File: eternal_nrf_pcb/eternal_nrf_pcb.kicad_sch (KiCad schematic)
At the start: 52 parts, among them J1 Conn_01x05_Pin, Q1 IRLML6244, Q2 IRLML6402, SW1 SW_Push, U1 BQ25504, U2 nRF52810-QCxx, U3 DRV5032DU, U4 SHTC3, Y1 Crystal_GND24

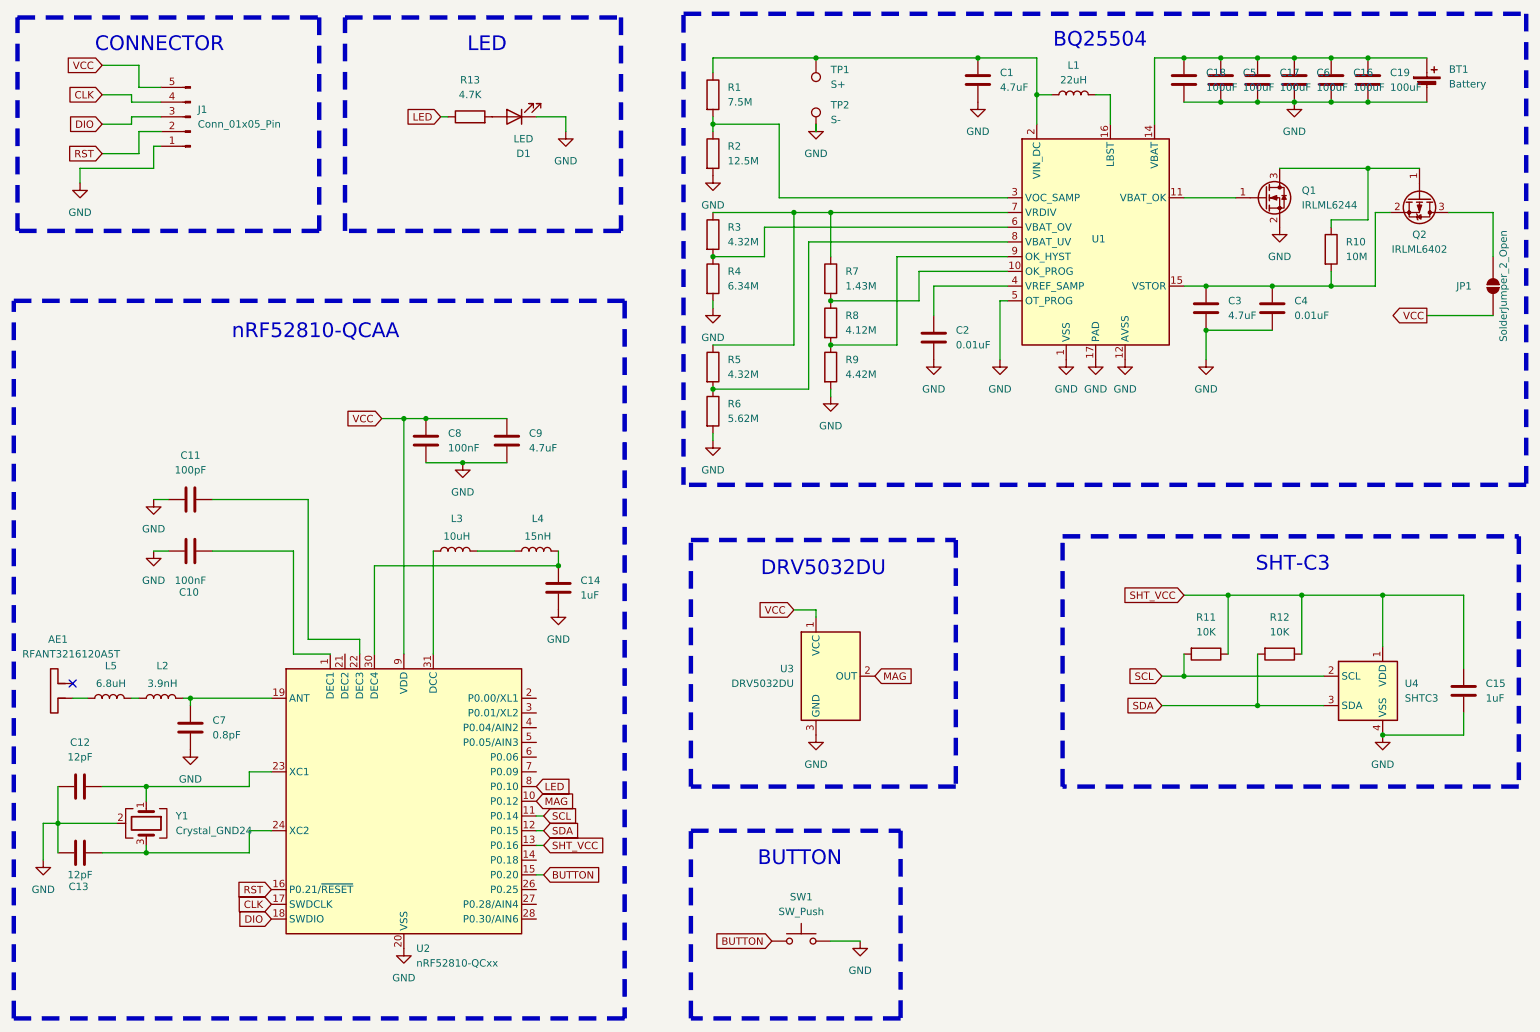
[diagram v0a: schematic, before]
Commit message: complete board
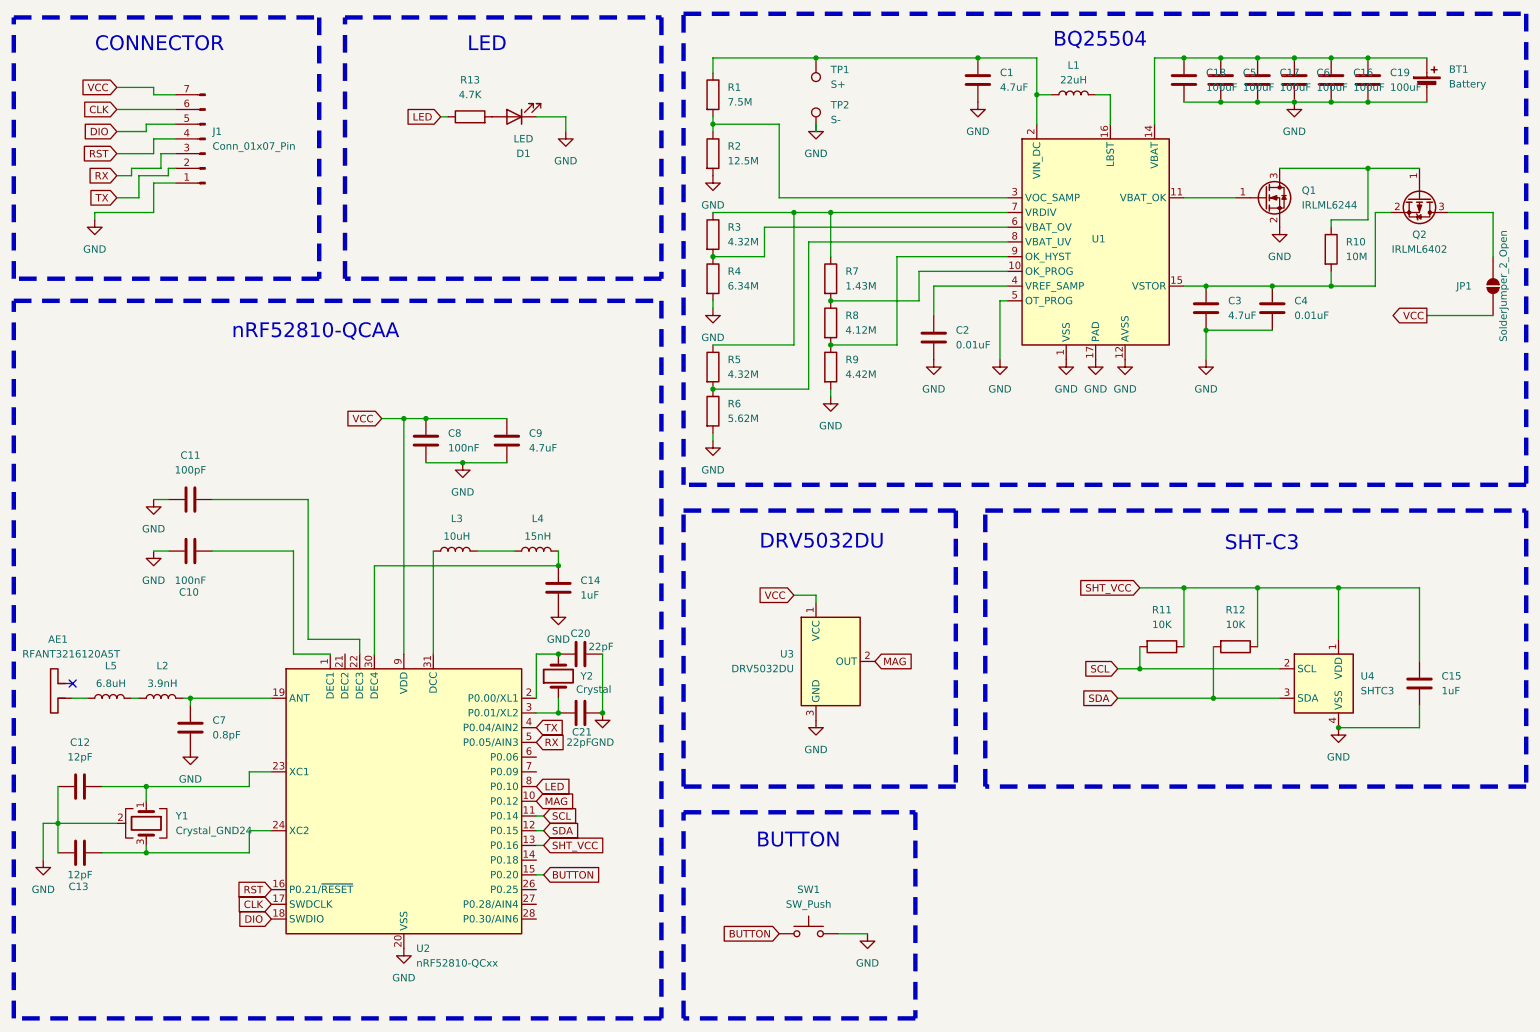
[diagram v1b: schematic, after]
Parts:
- removed J1: Conn_01x05_Pin, Connector_PinHeader_2.54mm:PinHeader_1x05_P2.54mm_Vertical, symbol Connector:Conn_01x05_Pin
- added C20, C21: 22pF, Capacitor_SMD:C_0402_1005Metric_Pad0.74x0.62mm_HandSolder, symbol Device:C
- added J1: Conn_01x07_Pin, Connector_PinHeader_2.54mm:PinHeader_1x07_P2.54mm_Vertical, symbol Connector:Conn_01x07_Pin
- added Y2: Crystal, Crystal:Crystal_SMD_3215-2Pin_3.2x1.5mm, symbol Device:Crystal
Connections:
- net CLK: now also J1.6 (Pin_6)
- net DIO: now also J1.5 (Pin_5)
- net GND: now also C20.1, C21.2, J1.1 (Pin_1)
- net RST: now also J1.4 (Pin_4)
- net VCC: now also J1.7 (Pin_7)
- net at U2.2 (P0.00/XL1): now also C21.1, Y2.2
- net at U2.3 (P0.01/XL2): now also C20.2, Y2.1
- net TX: now reaches U2.4 (P0.04/AIN2)
- net TX: now also J1.2 (Pin_2)
- net RX: now reaches U2.5 (P0.05/AIN3)
- net RX: now also J1.3 (Pin_3)
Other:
- moved on the sheet: C15, R11, R12, SW1, U3, U4
